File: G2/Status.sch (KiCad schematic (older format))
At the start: 47 parts, among them J601 Conn_02x08_Odd_Even, U601 TXB0102DCU

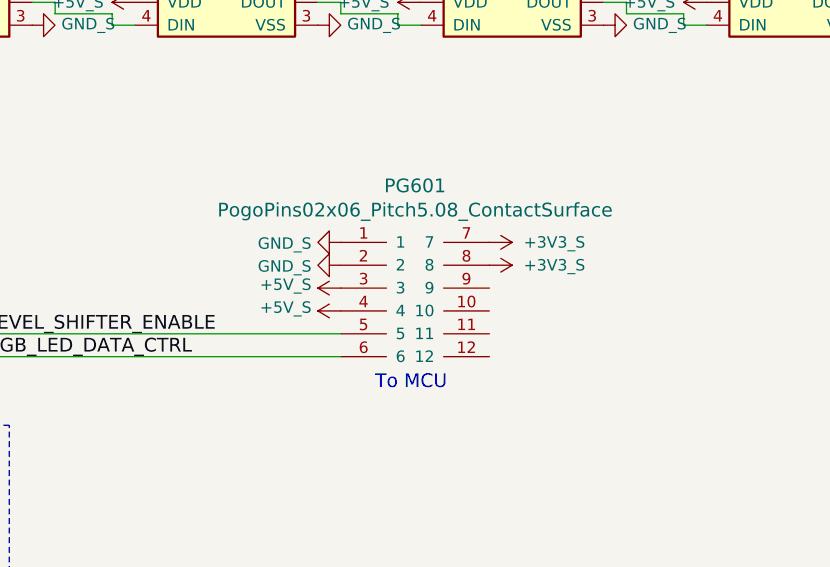
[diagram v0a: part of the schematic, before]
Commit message: No longer uses Pogo pins
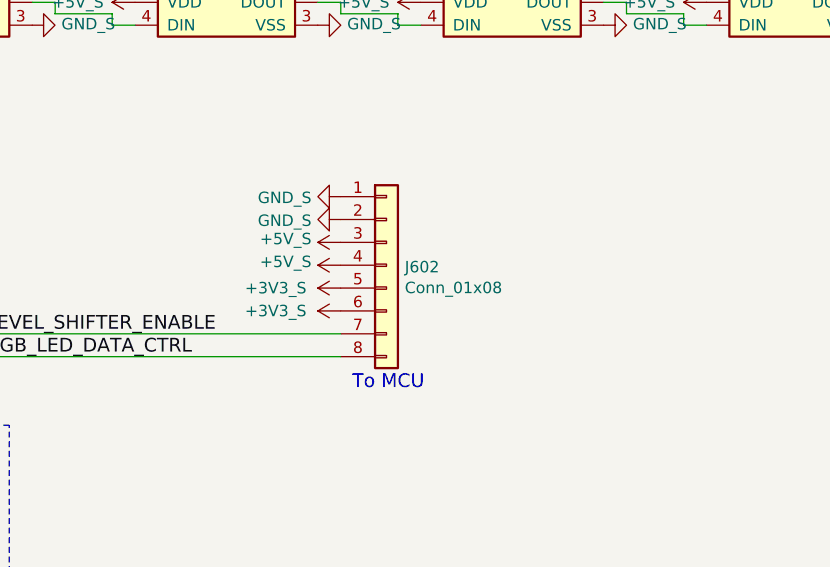
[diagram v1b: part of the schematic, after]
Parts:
- removed PG601: PogoPins02x06_Pitch5.08_ContactSurface, PogoPins02x06_Pitch5:PogoPins02x06_Pitch5.08_ContactSurface, symbol PogoPins02x06_Pitch5.08_ContactSurface
- added J602: Conn_01x08, LocalComponents:WE68710814022_8x0.50mm_SMT_ZIF_Horizontal_Top, symbol Conn_01x08
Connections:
- net +3V3_S: now also J602.5 (Pin_5), J602.6 (Pin_6)
- net +5V_S: now also J602.3 (Pin_3), J602.4 (Pin_4)
- net GND_S: now also J602.1 (Pin_1), J602.2 (Pin_2)
- net LEVEL_SHIFTER_ENABLE: now also J602.7 (Pin_7)
- net RGB_LED_DATA_CTRL: now also J602.8 (Pin_8)
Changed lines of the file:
@@
 L +3V3_S #PWR0130
 U 1 1 59CAE1C1
-P 6000 2450
-F 0 "#PWR0130" H 6000 2300 50  0001 C CNN
-F 1 "+3V3_S" V 6000 2600 50  0000 L CNN
-F 2 "" H 6000 2450 50  0001 C CNN
-F 3 "" H 6000 2450 50  0001 C CNN
-	1    6000 2450
-	0    1    1    0
+P 5350 2750
+F 0 "#PWR0130" H 5350 2600 50  0001 C CNN
+F 1 "+3V3_S" V 5350 2900 50  0000 L CNN
+F 2 "" H 5350 2750 50  0001 C CNN
+F 3 "" H 5350 2750 50  0001 C CNN
+	1    5350 2750
+	0    -1   -1   0
 $EndComp
 $Comp
 L GND_S #PWR0131
 U 1 1 59CAE2F4
+P 5350 2250
+F 0 "#PWR0131" H 5350 2000 50  0001 C CNN
+F 1 "GND_S" V 5355 2122 50  0000 R CNN
+F 2 "" H 5350 2250 50  0001 C CNN
+F 3 "" H 5350 2250 50  0001 C CNN
+	1    5350 2250
+	0    1    1    0
+$EndComp
+$Comp
+L +3V3_S #PWR0132
+U 1 1 59CAE368
+P 5350 2650
+F 0 "#PWR0132" H 5350 2500 50  0001 C CNN
+F 1 "+3V3_S" V 5350 2800 50  0000 L CNN
+F 2 "" H 5350 2650 50  0001 C CNN
+F 3 "" H 5350 2650 50  0001 C CNN
+	1    5350 2650
+	0    -1   -1   0
+$EndComp
+$Comp
+L GND_S #PWR0133
+U 1 1 59CAE815
+P 5350 2350
+F 0 "#PWR0133" H 5350 2100 50  0001 C CNN
+F 1 "GND_S" V 5355 2222 50  0000 R CNN
+F 2 "" H 5350 2350 50  0001 C CNN
+F 3 "" H 5350 2350 50  0001 C CNN
+	1    5350 2350
+	0    1    1    0
+$EndComp
+$Comp
+L +5V_S #PWR0134
+U 1 1 59CAED7D
 P 5350 2450
-F 0 "#PWR0131" H 5350 2200 50  0001 C CNN
-F 1 "GND_S" V 5355 2322 50  0000 R CNN
+F 0 "#PWR0134" H 5350 2300 50  0001 C CNN
+F 1 "+5V_S" V 5365 2578 50  0000 L CNN
 F 2 "" H 5350 2450 50  0001 C CNN
 F 3 "" H 5350 2450 50  0001 C CNN
 	1    5350 2450
-	0    1    1    0
-$EndComp
-$Comp
-L +3V3_S #PWR0132
-U 1 1 59CAE368
-P 6000 2550
-F 0 "#PWR0132" H 6000 2400 50  0001 C CNN
-F 1 "+3V3_S" V 6000 2700 50  0000 L CNN
-F 2 "" H 6000 2550 50  0001 C CNN
-F 3 "" H 6000 2550 50  0001 C CNN
-	1    6000 2550
-	0    1    1    0
-$EndComp
-$Comp
-L GND_S #PWR0133
-U 1 1 59CAE815
+	0    -1   -1   0
+$EndComp
+$Comp
+L +5V_S #PWR0135
+U 1 1 59CAEEB5
 P 5350 2550
-F 0 "#PWR0133" H 5350 2300 50  0001 C CNN
-F 1 "GND_S" V 5355 2422 50  0000 R CNN
+F 0 "#PWR0135" H 5350 2400 50  0001 C CNN
+F 1 "+5V_S" V 5365 2678 50  0000 L CNN
 F 2 "" H 5350 2550 50  0001 C CNN
 F 3 "" H 5350 2550 50  0001 C CNN
 	1    5350 2550
-	0    1    1    0
-$EndComp
-$Comp
-L +5V_S #PWR0134
-U 1 1 59CAED7D
-P 5350 2650
-F 0 "#PWR0134" H 5350 2500 50  0001 C CNN
-F 1 "+5V_S" V 5365 2778 50  0000 L CNN
-F 2 "" H 5350 2650 50  0001 C CNN
-F 3 "" H 5350 2650 50  0001 C CNN
-	1    5350 2650
-	0    -1   -1   0
-$EndComp
-$Comp
-L +5V_S #PWR0135
-U 1 1 59CAEEB5
-P 5350 2750
-F 0 "#PWR0135" H 5350 2600 50  0001 C CNN
-F 1 "+5V_S" V 5365 2878 50  0000 L CNN
-F 2 "" H 5350 2750 50  0001 C CNN
-F 3 "" H 5350 2750 50  0001 C CNN
-	1    5350 2750
 	0    -1   -1   0
 $EndComp
@@
 	1    0    0    -1
 $EndComp
-Text Notes 5500 3100 0    60   ~ 0
+Text Notes 5400 3100 0    60   ~ 0
 To MCU
 Wire Wire Line
@@
 	1    0    0    -1
 $EndComp
-$Comp
-L PogoPins02x06_Pitch5.08_ContactSurface PG601
-U 1 1 59CF7341
-P 5550 2350
-F 0 "PG601" H 5675 2497 60  0000 C CNN
-F 1 "PogoPins02x06_Pitch5.08_ContactSurface" H 5675 2391 60  0000 C CNN
-F 2 "PogoPins02x06_Pitch5:PogoPins02x06_Pitch5.08_ContactSurface" H 5550 2350 60  0001 C CNN
-F 3 "" H 5550 2350 60  0001 C CNN
-	1    5550 2350
-	1    0    0    -1
-$EndComp
 Wire Wire Line
 	3200 1500 3200 1700
@@
 Wire Wire Line
 	1550 1700 1650 1700
+$Comp
+L Conn_01x08 J602
+U 1 1 5A080018
+P 5550 2550
+F 0 "J602" H 5630 2542 50  0000 L CNN
+F 1 "Conn_01x08" H 5630 2451 50  0000 L CNN
+F 2 "LocalComponents:WE68710814022_8x0.50mm_SMT_ZIF_Horizontal_Top" H 5550 2550 50  0001 C CNN
+F 3 "https://www.mouser.se/Search/ProductDetail.aspx?qs=ZtY9WdtwX54hJHBraEAPJw%3d%3d" H 5550 2550 50  0001 C CNN
+	1    5550 2550
+	1    0    0    -1
+$EndComp
 $EndSCHEMATC
